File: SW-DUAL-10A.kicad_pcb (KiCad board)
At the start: 2 copper layers, 100 x 74 mm, 26 parts, among them J1 SW1, J2 SW2, J3 GND +SW1, J4 GND +SW2, J5 GND +12V, U1 BTS7002-1EPP, U2 BTS7002-1EPP

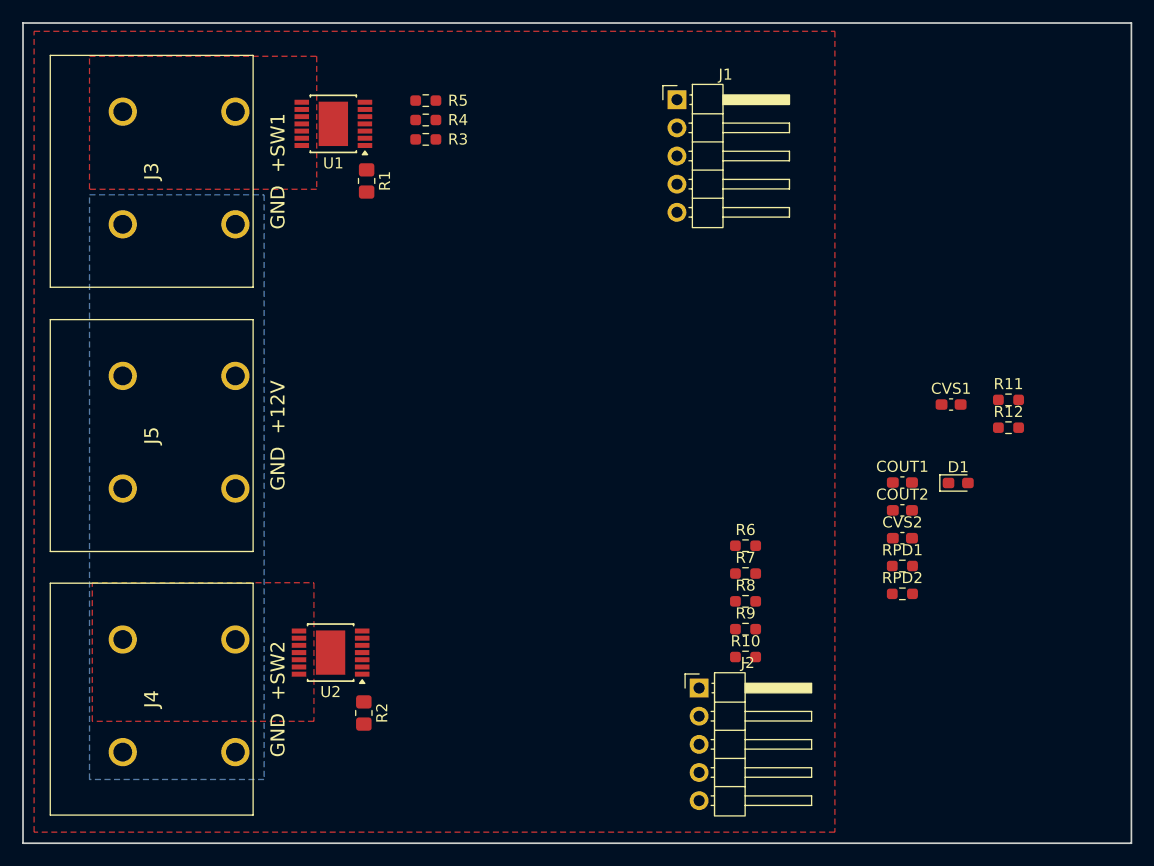
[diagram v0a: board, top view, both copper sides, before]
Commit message: everything is on the layout, needs a lot of tuning
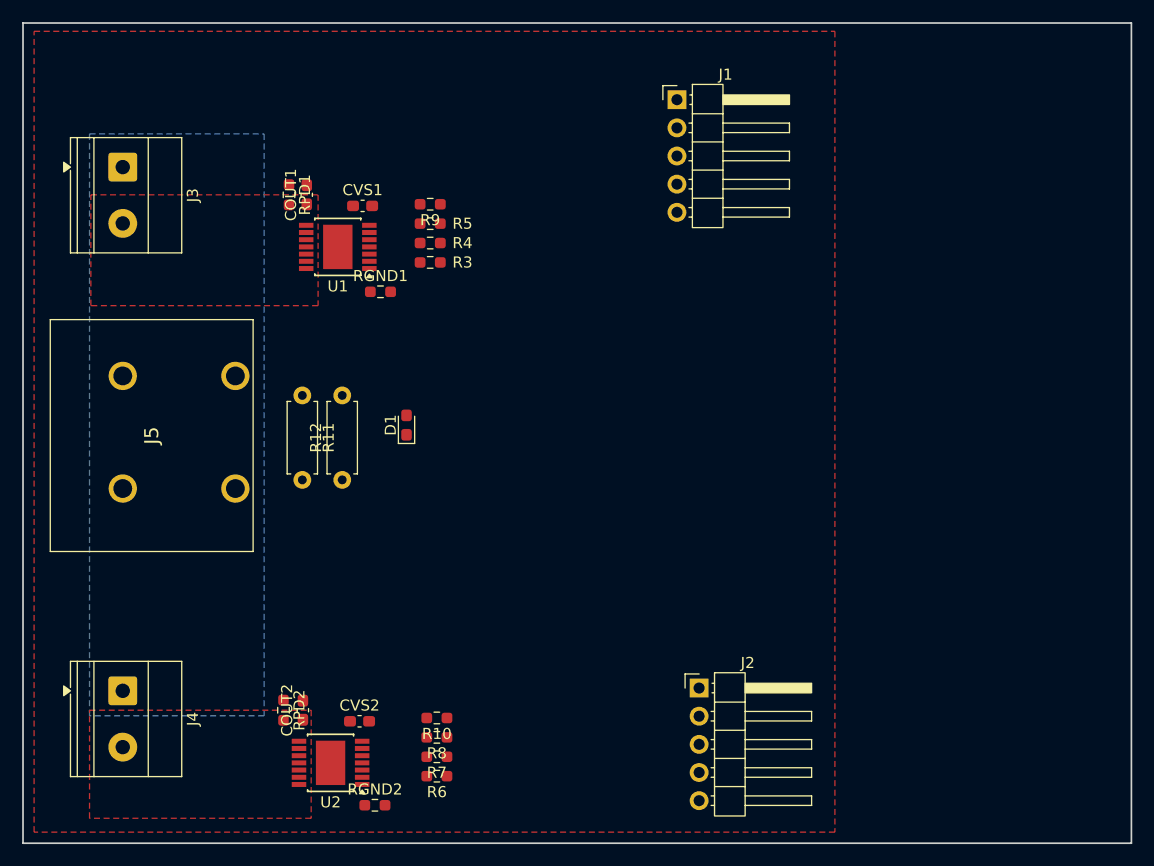
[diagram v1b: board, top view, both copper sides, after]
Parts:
- J3: value GND +SW1 -> Screw_Terminal_01x02; footprint SamacSys_Parts:VP0265840000G -> TerminalBlock_Phoenix:TerminalBlock_Phoenix_MKDS-1,5-2-5.08_1x02_P5.08mm_Horizontal
- J4: value GND +SW2 -> Screw_Terminal_01x02; footprint SamacSys_Parts:VP0265840000G -> TerminalBlock_Phoenix:TerminalBlock_Phoenix_MKDS-1,5-2-5.08_1x02_P5.08mm_Horizontal
- J5: value GND +12V -> PWRIN
- R11, R12: footprint Resistor_SMD:R_0603_1608Metric_Pad0.98x0.95mm_HandSolder -> Resistor_THT:R_Axial_DIN0207_L6.3mm_D2.5mm_P7.62mm_Horizontal
- RGND1: renamed from R1; footprint Resistor_SMD:R_0805_2012Metric_Pad1.20x1.40mm_HandSolder -> Resistor_SMD:R_0603_1608Metric_Pad0.98x0.95mm_HandSolder
- RGND2: renamed from R2; footprint Resistor_SMD:R_0805_2012Metric_Pad1.20x1.40mm_HandSolder -> Resistor_SMD:R_0603_1608Metric_Pad0.98x0.95mm_HandSolder
- moved RPD1 64.7 mm to (114.0, 81.5), turned to -90 degrees
- moved R11 63.7 mm to (115.2, 99.6), turned to -90 degrees
- moved R12 60.3 mm to (118.8, 107.2), turned to 90 degrees
- moved COUT1 59.7 mm to (115.6, 81.5), turned to 90 degrees
- moved COUT2 57.0 mm to (115.2, 128.0), turned to 90 degrees
- moved RPD2 56.8 mm to (113.5, 128.0), turned to -90 degrees
- moved CVS1 56.0 mm to (120.6, 82.5)
- moved CVS2 51.7 mm to (120.4, 129.0)
- moved D1 50.0 mm to (124.6, 102.3), turned to 90 degrees
- moved R9 47.7 mm to (126.7, 82.3), turned to 180 degrees
- moved R6 34.8 mm to (127.3, 133.9), turned to 180 degrees
- moved R7 32.4 mm to (127.3, 132.2), turned to 180 degrees
- moved R8 30.4 mm to (127.3, 130.4), turned to 180 degrees
- moved R10 28.4 mm to (127.3, 128.7), turned to 180 degrees
- moved U1 11.1 mm to (118.4, 86.2)
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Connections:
- J3 pad 1: /SW1OUT -> GND
- J4 pad 1: /SW2OUT -> GND
